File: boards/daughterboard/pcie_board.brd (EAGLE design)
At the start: 97.3 x 93 mm, 61 parts, among them IC1 XMEGA16A4A, IC2 SN754410, T1 2N3704, T2 2N3704, T3 2N3704, T4 2N3704, T5 2N3704, T6 2N3704, T7 2N3704, X1 PCI-E1X_EDGE

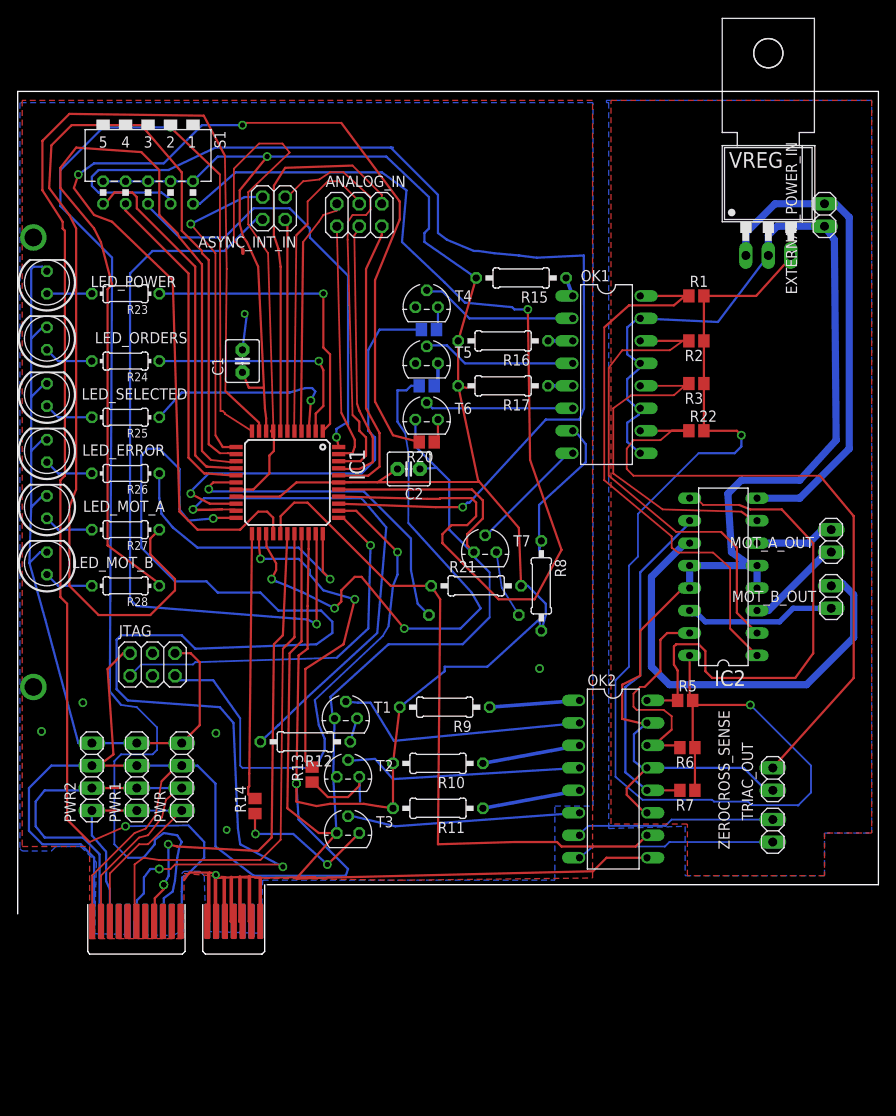
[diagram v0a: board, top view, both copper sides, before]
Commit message: Latest board(the one presented at class
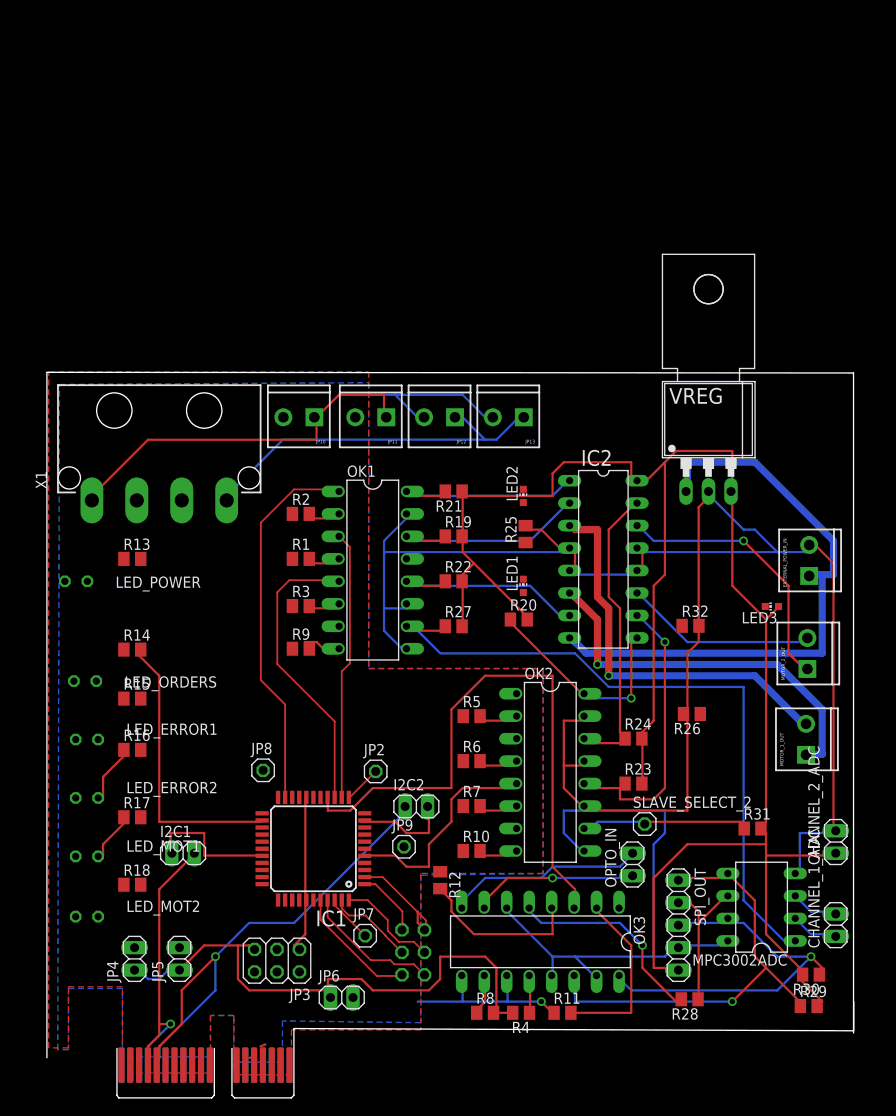
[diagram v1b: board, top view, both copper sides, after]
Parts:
- removed ANALOG_IN, JTAG: (no value), pinhead:2X03
- removed ASYNC_INT_IN: (no value), pinhead:2X02
- removed C1, C2: (no value), capacitor-wima:C2.5-4
- removed LED_ERROR, LED_MOT_A, LED_MOT_B, LED_SELECTED: (no value), led:LED5MM
- removed MOT_A_OUT, MOT_B_OUT, TRIAC_OUT, ZEROCROSS_SENSE: (no value), pinhead:1X02
- removed PWR, PWR1, PWR2: (no value), pinhead:1X04
- removed S1: (no value), switch-dil:DA-05
- removed T1, T2, T3, T4, T5, T6, T7: 2N3704, transistor:TO92
- added CHANNEL_1_ADC, CHANNEL_2_ADC, I2C1, I2C2, JP4, JP5, JP6, OPTO_IN: (no value), pinhead:1X02
- added JP1, JP3: (no value), pinhead:2X03
- added JP10, JP11, JP12, JP13, MOTOR_1_OUT, MOTOR_2_OUT: (no value), SparkFun:SCREWTERMINAL-3.5MM-2
- added JP2, JP7, JP8, JP9, SLAVE_SELECT_2: (no value), pinhead:1X01
- added LED1, LED2, LED3: (no value), led:CHIP-LED0603
- added LED_ERROR1, LED_ERROR2, LED_MOT1, LED_MOT2: (no value), led:LED5MM
- added MPC3002ADC: (no value), ic-package:DIL08
- added OK3: TIL193, optocoupler:DIL16
- added R29, R30, R31, R32: (no value), resistor:M0805
- added SPI_OUT: (no value), pinhead:1X05
- added U$1: PCI-E1X_EDGE, con-pci_express(pci-e):PCI-E_X1_EDGE
- EXTERNAL_POWER_IN: device pinhead:1X02 -> SparkFun:SCREWTERMINAL-3.5MM-2
- OK1, OK2: value ILQ620 -> TIL193
- R1, R2, R22, R3, R5, R6, R7: value 10K -> (none); device resistor:R0805 -> resistor:M0805
- R10, R11, R15, R16, R17, R8, R9: value 47Ohm -> (none); device resistor:0207/10 -> resistor:M0805
- R12, R4: value 100Ohm -> (none); device resistor:0207/10 -> resistor:M0805
- R13, R14, R18, R19, R20: value 100Ohm -> (none); device resistor:R0805 -> resistor:M0805
- R21: value 10K -> (none); device resistor:0207/10 -> resistor:M0805
- R23, R24, R25, R26, R27, R28: value 47Ohm -> (none); device resistor:0204/7 -> resistor:M0805
- X1: value PCI-E1X_EDGE -> 9090-4R; device con-pci_express(pci-e):PCI-E_X1_EDGE -> con-thomas-betts:9090-4R
- moved R23 79.8 mm to (66.3, 23.4), turned to 0 degrees
- moved R28 79.0 mm to (72.6, -1.02)
- moved R24 71.5 mm to (66.3, 28.4), turned to 0 degrees
- moved R18 71.1 mm to (9.65, 11.9), flipped to the top
- moved R26 69.5 mm to (72.9, 31.2)
- moved R15 64.7 mm to (9.65, 33.0), turned to 0 degrees
- moved R17 64.3 mm to (9.65, 19.6), turned to 0 degrees
- moved R16 62.4 mm to (9.65, 27.2), turned to 0 degrees
- moved R1 53.7 mm to (28.7, 48.8)
- moved X1 52.4 mm to (12.7, 61.7)
- moved R3 51.3 mm to (28.7, 43.4), turned to 0 degrees
- moved R2 48.8 mm to (28.7, 53.8), turned to 0 degrees
- moved R8 48.7 mm to (49.5, -2.54), turned to 0 degrees
- moved R25 47.1 mm to (54.1, 51.6), turned to 90 degrees
- moved R4 45.3 mm to (53.6, -2.54), flipped to the top, turned to 180 degrees
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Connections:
- removed net +12V: PWR.1, PWR1.1, PWR2.1, X1.A3, X1.B3
- removed net +5V: PWR.2, PWR1.2, PWR2.2, X1.A2, X1.B2
- removed net EXT_5V: IC2.16, R1.2, R2.1, R22.2, R3.1, R5.2, R6.1, R7.1, VREG.OUT
- removed net N$15: IC1.13, R27.1
- removed net N$4: LED_POWER.A, R23.2
- removed net N$43: IC2.14, MOT_B_OUT.1
- removed net N$45: IC1.16, S1.7
- removed net N$46: IC1.15, S1.6
- removed net N$47: OK2.3, R10.1
- removed net N$48: OK2.5, R11.1
- removed net N$49: OK2.4, T2.2
- removed net N$50: OK2.6, T3.2
- removed net N$51: R12.1, T1.1
- removed net N$52: R13.1, T2.1
- removed net N$53: R14.1, T3.1
- removed net N$55: IC1.23, R14.2
- removed net N$56: IC1.24, R13.2
- removed net N$57: OK1.2, T4.2
- removed net N$58: OK1.4, T5.2
- removed net N$59: OK1.6, T6.2
- removed net N$60: R18.1, T4.1
- removed net N$61: R19.1, T5.1
- removed net N$62: R20.1, T6.1
- removed net N$65: IC1.25, R19.2
- removed net N$66: IC1.26, R20.2
- removed net N$67: OK1.1, R15.1
- removed net N$68: OK1.3, R16.1
- removed net N$69: OK1.5, R17.1
- removed net N$70: IC1.44, S1.8
- removed net N$71: ANALOG_IN.2, IC1.4
- removed net N$73: ANALOG_IN.5, IC1.40
- removed net N$74: ANALOG_IN.3, IC1.41
- removed net N$75: ASYNC_INT_IN.1, IC1.42
- removed net N$77: IC1.1, R23.1
- removed net PWM_A: IC1.21, R12.2
- removed net TRIAC_OUT: IC1.17, R4.2
- removed net ZEROCROSS_IN: IC1.27, OK2.10, R21.1
- new net ADC_CLK: MPC3002ADC.7, OK3.16, R30.1, SPI_OUT.3
- new net ADC_CS: MPC3002ADC.1, OK1.10, R27.1
- new net ADC_MISO: MPC3002ADC.6, R28.1, SPI_OUT.2
- new net ADC_MOSI: MPC3002ADC.5, OK3.14, R29.1, SPI_OUT.1
- new net ADC_VSS: CHANNEL_2_ADC.1, IC2.16, LED3.A, R19.2, R20.2, R21.1, R22.2, R23.2, R24.2, R27.2, R29.2, R30.2, R31.2, SPI_OUT.5, VREG.OUT
- new net ANALOG_1: IC1.40, JP1.1
- new net ANALOG_2: IC1.41, JP1.2
- new net ANALOG_3: IC1.43, JP1.3
- new net ANALOG_4: IC1.44, JP1.4
- new net ANALOG_5: IC1.1, JP1.5
- new net ANALOG_6: IC1.2, JP1.6
- new net ASYNC_1: IC1.22, JP8.1
- new net ASYNC_2: IC1.12, JP2.1
- new net ASYNC_3: IC1.6, JP9.1
- new net ASYNC_4: IC1.42, JP7.1
- new net CHANNEL_1: CHANNEL_1_ADC.1, MPC3002ADC.2
- new net LED_ERROR1: IC1.25, R15.2
- new net LED_ERROR2: IC1.26, R16.2
- new net LED_MOT_1: IC1.27, R17.2
- new net LED_MOT_2: IC1.33, R18.2
- new net LED_ORDERS: IC1.24, R14.2
- new net LED_POWER: IC1.23, R13.2
- new net MISO: IC1.16, OK3.12, R4.1
- new net MOSI: IC1.15, OK3.3
- new net MOT_CONTROL_A_1: IC1.13, OK1.3
- new net MOT_CONTROL_A_2: IC1.7, OK2.3
- new net MOT_CONTROL_B_1: IC1.14, OK1.5
- new net MOT_CONTROL_B_2: IC1.5, OK2.5
- new net MOT_CONTROL_EN_1: IC1.21, OK1.1
- new net MOT_CONTROL_EN_2: IC1.20, OK2.1
- new net N$38: JP10.1, JP11.1, X1.1
- new net OPTIONAL_OPTO_IN: OK3.10, R8.1
- new net PDI_CLK: IC1.35, JP3.2
- new net PDI_DATA: IC1.34, JP3.6
- new net SCK: IC1.17, OK3.1
- new net SS1: IC1.3, OK2.7
- new net SS2: IC1.4, OK1.7
- net +3V3: now also JP3.5, JP4.1, JP5.1, JP6.1, R4.2, U$1.A1, U$1.A2, U$1.B1, U$1.B2; no longer C1.1, C2.2, JTAG.2, PWR.3, PWR1.3, PWR2.3, R10.2, R11.2, R15.2, R16.2, R17.2, R21.2, R9.2, S1.1, S1.2, S1.3, S1.4, S1.5, X1.A1, X1.B1
- net ERROR: now also IC1.32, U$1.A7, U$1.B7; no longer IC1.22, X1.A6
- net EXT_MOTOR_GND: now also CHANNEL_2_ADC.2, MPC3002ADC.4, MPC3002ADC.8, OK2.9, OK3.13, OK3.15, OK3.6, R25.2, R26.2, R32.2, SPI_OUT.4; no longer TRIAC_OUT.2
- net GND: now also JP10.2, JP11.2, JP12.2, JP13.2, JP3.1, JP4.2, JP5.2, LED_ERROR1.K, LED_ERROR2.K, LED_MOT1.K, LED_MOT2.K, OK3.11, OK3.9, R1.1, R10.1, R11.1, R12.1, R2.1, R3.1, R5.1, R6.1, R7.1, R9.1, U$1.A10, U$1.A11, U$1.A12, U$1.A13, U$1.A14, U$1.A15, U$1.A16, U$1.A17, U$1.A18, U$1.A8, U$1.A9, U$1.B10, U$1.B11, U$1.B12, U$1.B13, U$1.B14, U$1.B15, U$1.B16, U$1.B17, U$1.B18, U$1.B8, U$1.B9, X1.2, X1.3; no longer C1.2, C2.1, JTAG.6, LED_ERROR.K, LED_MOT_A.K, LED_MOT_B.K, LED_SELECTED.K, OK2.9, PWR.4, PWR1.4, PWR2.4, T1.3, T2.3, T3.3, T4.3, T5.3, T6.3, T7.3, X1.A10, X1.A12, X1.A13, X1.A14, X1.A15, X1.A16, X1.A17, X1.A18, X1.A4, X1.A5, X1.A7, X1.A8, X1.B10, X1.B11, X1.B12, X1.B13, X1.B14, X1.B15, X1.B16, X1.B17, X1.B18, X1.B4, X1.B5, X1.B7, X1.B9
- net N$1: now also IC2.14, MOTOR_2_OUT.1; no longer IC1.3, R25.1
- net N$10: now also OK2.4, R6.2; no longer IC1.33, R26.1
- net N$11: now also OK2.6, R7.2; no longer LED_ERROR.A, R26.2
- net N$12: now also OK2.8, R10.2; no longer ANALOG_IN.4, IC1.5
- net N$13: now also OK3.2, R11.2; no longer ANALOG_IN.6, IC1.7
- net N$14: now also OK3.4, R12.2; no longer ASYNC_INT_IN.3, IC1.12
- net N$16: now also LED_POWER.A, R13.1; no longer ANALOG_IN.1, IC1.43
- net N$17: now also LED_ORDERS.A, R14.1; no longer IC1.14, R28.1
- net N$18: now also CHANNEL_1_ADC.2, MPC3002ADC.3; no longer ASYNC_INT_IN.4, IC1.32
- net N$19: now also OK2.10, R31.1, SLAVE_SELECT_2.1; no longer LED_MOT_B.A, R28.2
- net N$2: now also JP12.1, JP13.1, X1.4; no longer IC1.35, JTAG.5
- net N$20: now also LED_ERROR1.A, R15.1; no longer IC1.2, R24.1
- net N$21: now also LED_ERROR2.A, R16.1; no longer ASYNC_INT_IN.2, IC1.6
- net N$22: now also LED_MOT1.A, R17.1; no longer LED_MOT_A.A, R27.2
- net N$23: now also LED_MOT2.A, R18.1; no longer IC1.36, S1.9
- net N$24: now also IC2.1, LED2.A, OK1.16, R21.2; no longer IC1.37, S1.10
- net N$25: now also IC2.2, OK1.14, R19.1; no longer OK1.8, T7.2
- net N$26: now also LED2.C, R25.1; no longer JTAG.3
- net N$27: now also LED1.C, R26.1; no longer JTAG.4
- net N$28: now also IC2.9, LED1.A, OK2.16, R20.1; no longer OK2.7, ZEROCROSS_SENSE.1
- net N$29: now also IC2.7, OK1.12, R22.1; no longer OK2.2, T1.2
- net N$3: now also IC2.11, MOTOR_2_OUT.2; no longer R4.1, T7.1
- net N$30: now also IC2.15, OK2.14, R24.1; no longer OK2.1, R9.1
- net N$31: now also MOTOR_1_OUT.2; no longer MOT_A_OUT.2
- net N$32: now also MOTOR_1_OUT.1; no longer MOT_A_OUT.1
- net N$33: now also IC2.10, OK2.12, R23.1; no longer IC2.1, OK1.16, R1.1
- net N$34: now also OK3.5, R28.2; no longer IC2.2, OK1.14, R2.2
- net N$35: now also OK3.7, OPTO_IN.1; no longer IC2.7, OK1.12, R3.2
- net N$36: now also OK3.8, OPTO_IN.2; no longer OK2.8, ZEROCROSS_SENSE.2
- net N$37: now also LED3.C, R32.1; no longer IC1.20, R18.2
- net N$39: now also JP3.4; no longer IC2.11, MOT_B_OUT.2
- net N$40: now also JP3.3; no longer IC2.9, OK2.16, R5.1
- net N$41: now also IC1.36; no longer IC2.15, OK2.14, R6.2
- net N$42: now also IC1.37, JP6.2; no longer IC2.10, OK2.12, R7.2
- net N$5: now also OK1.2, R2.2; no longer OK1.10, R22.1, TRIAC_OUT.1
- net N$6: now also OK1.4, R1.2; no longer LED_ORDERS.A, R24.2
- net N$7: now also OK1.6, R3.2; no longer LED_SELECTED.A, R25.2
- net N$8: now also OK1.8, R9.2; no longer OK1.7, R8.1
- net N$9: now also OK2.2, R5.2; no longer IC1.34, JTAG.1
- net SCL1: now also I2C1.1, U$1.A3, U$1.B3; no longer X1.B6
- net SCL2: now also I2C2.1, U$1.A5, U$1.B5; no longer X1.A9
- net SDA1: now also I2C1.2, U$1.A4, U$1.B4; no longer X1.B8
- net SDA2: now also I2C2.2, U$1.A6, U$1.B6; no longer X1.A11
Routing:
- net GND: track 388.0 -> 60.6 mm, vias 3 -> 1
- net +3V3: track 381.3 -> 63.1 mm, vias 4 -> 0
- net ADC_VSS: track 0.00 -> 206.2 mm
- net SDA2: track 161.6 -> 11.6 mm, vias 1 -> 0
- net ERROR: track 140.7 -> 0.00 mm, vias 3 -> 0
- net EXT_5V: track 138.3 -> 0.00 mm, vias 2 -> 0
- net N$66: track 131.2 -> 0.00 mm, vias 2 -> 0
- net N$15: track 127.4 -> 0.00 mm
- net N$23: track 124.8 -> 0.00 mm, vias 1 -> 0
- net EXT_MOTOR_GND: track 160.7 -> 281.3 mm
- net N$17: track 103.4 -> 0.00 mm
- net SCL2: track 158.6 -> 58.8 mm
- net N$24: track 119.3 -> 24.7 mm, vias 1 -> 0
- net N$18: track 86.6 -> 5.41 mm, vias 1 -> 0
- net ADC_CS: track 0.00 -> 78.6 mm
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- removed copper zone on layer 1, net EXT_MOTOR_GND
- removed copper zone on layer 16, net EXT_MOTOR_GND
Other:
- board size 97.3 x 93 mm -> 91.2 x 77.5 mm
